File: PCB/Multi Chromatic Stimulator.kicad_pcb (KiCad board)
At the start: 2 copper layers, 125 x 75 mm, 38 parts, among them J2 5V - 30V

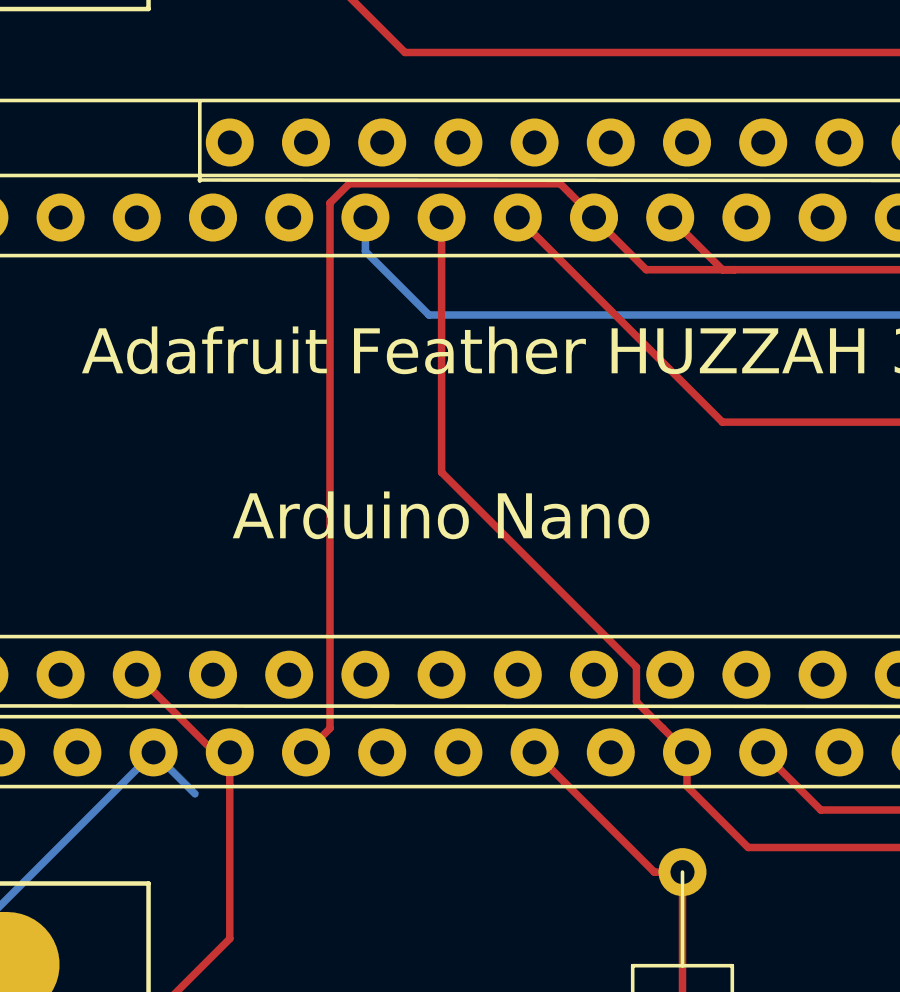
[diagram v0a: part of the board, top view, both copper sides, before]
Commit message: v2.1
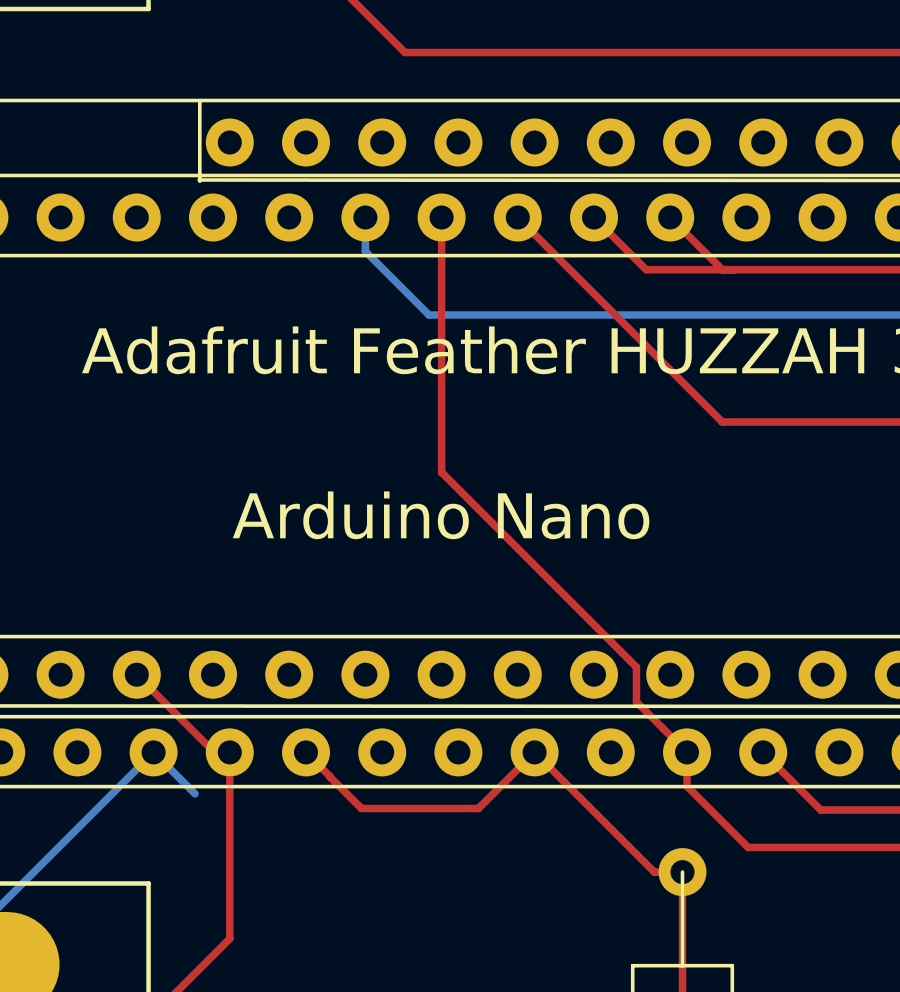
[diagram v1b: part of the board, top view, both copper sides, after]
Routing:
- net Net-(A1-Pad23): track 194.1 -> 175.1 mm
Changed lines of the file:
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@@
     (thickness 1.6)
     (drawings 87)
-    (tracks 279)
+    (tracks 278)
     (zones 0)
     (modules 38)
@@
     (effects (font (size 1.5 1.5) (thickness 0.3)))
   )
-  (segment (start 146.5 70.665) (end 146.955 71.12) (width 0.25) (layer F.Cu) (net 38))
   (segment (start 77.41 101.04116) (end 77.41 94.83) (width 0.25) (layer F.Cu) (net 2))
   (segment (start 72.50126 107) (end 72.50126 105.9499) (width 0.25) (layer F.Cu) (net 2))
@@
   (segment (start 92.5 103.25) (end 91.630001 104.119999) (width 0.25) (layer F.Cu) (net 6))
   (segment (start 92.5 98.82) (end 92.5 103.25) (width 0.25) (layer F.Cu) (net 6))
-  (segment (start 88.750001 76.200001) (end 89.55 77) (width 0.25) (layer F.Cu) (net 6))
-  (segment (start 88.424999 75.874999) (end 88.750001 76.200001) (width 0.25) (layer F.Cu) (net 6))
-  (segment (start 81.389999 75.874999) (end 88.424999 75.874999) (width 0.25) (layer F.Cu) (net 6))
-  (segment (start 80.749999 76.514999) (end 81.389999 75.874999) (width 0.25) (layer F.Cu) (net 6))
-  (segment (start 80.749999 94.030001) (end 80.749999 76.514999) (width 0.25) (layer F.Cu) (net 6))
-  (segment (start 79.95 94.83) (end 80.749999 94.030001) (width 0.25) (layer F.Cu) (net 6))
   (segment (start 93.83 78.74) (end 94.25 78.74) (width 0.25) (layer F.Cu) (net 6))
   (segment (start 92.09 77) (end 93.83 78.74) (width 0.25) (layer F.Cu) (net 6))
   (segment (start 91.29 78.74) (end 94.25 78.74) (width 0.25) (layer F.Cu) (net 6))
   (segment (start 94.25 78.74) (end 104 78.74) (width 0.25) (layer F.Cu) (net 6))
+  (segment (start 85.7 96.7) (end 87.57 94.83) (width 0.25) (layer F.Cu) (net 6))
+  (segment (start 81.8 96.7) (end 85.7 96.7) (width 0.25) (layer F.Cu) (net 6))
+  (segment (start 80.749999 95.649999) (end 81.8 96.7) (width 0.25) (layer F.Cu) (net 6))
+  (segment (start 79.95 94.83) (end 80.749999 95.629999) (width 0.25) (layer F.Cu) (net 6))
+  (segment (start 80.749999 95.629999) (end 80.749999 95.649999) (width 0.25) (layer F.Cu) (net 6))
   (segment (start 91.850001 94.030001) (end 92.65 94.83) (width 0.25) (layer F.Cu) (net 8))
   (segment (start 90.964999 93.144999) (end 91.850001 94.030001) (width 0.25) (layer F.Cu) (net 8))
@@
   (segment (start 105.185 54.75) (end 124.095 73.66) (width 0.25) (layer B.Cu) (net 37))
   (segment (start 76.625 54.75) (end 105.185 54.75) (width 0.25) (layer B.Cu) (net 37))
+  (segment (start 146.5 70.665) (end 146.955 71.12) (width 0.25) (layer F.Cu) (net 38))
   (segment (start 179.775 91.5) (end 181 91.5) (width 1) (layer F.Cu) (net 38))
   (segment (start 172.775 84.5) (end 179.775 91.5) (width 1) (layer F.Cu) (net 38))
